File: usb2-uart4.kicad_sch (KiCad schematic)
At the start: 20 parts, among them U1 CH344Q, U13 TPNUP2202W1T2G, Y1 8MHz

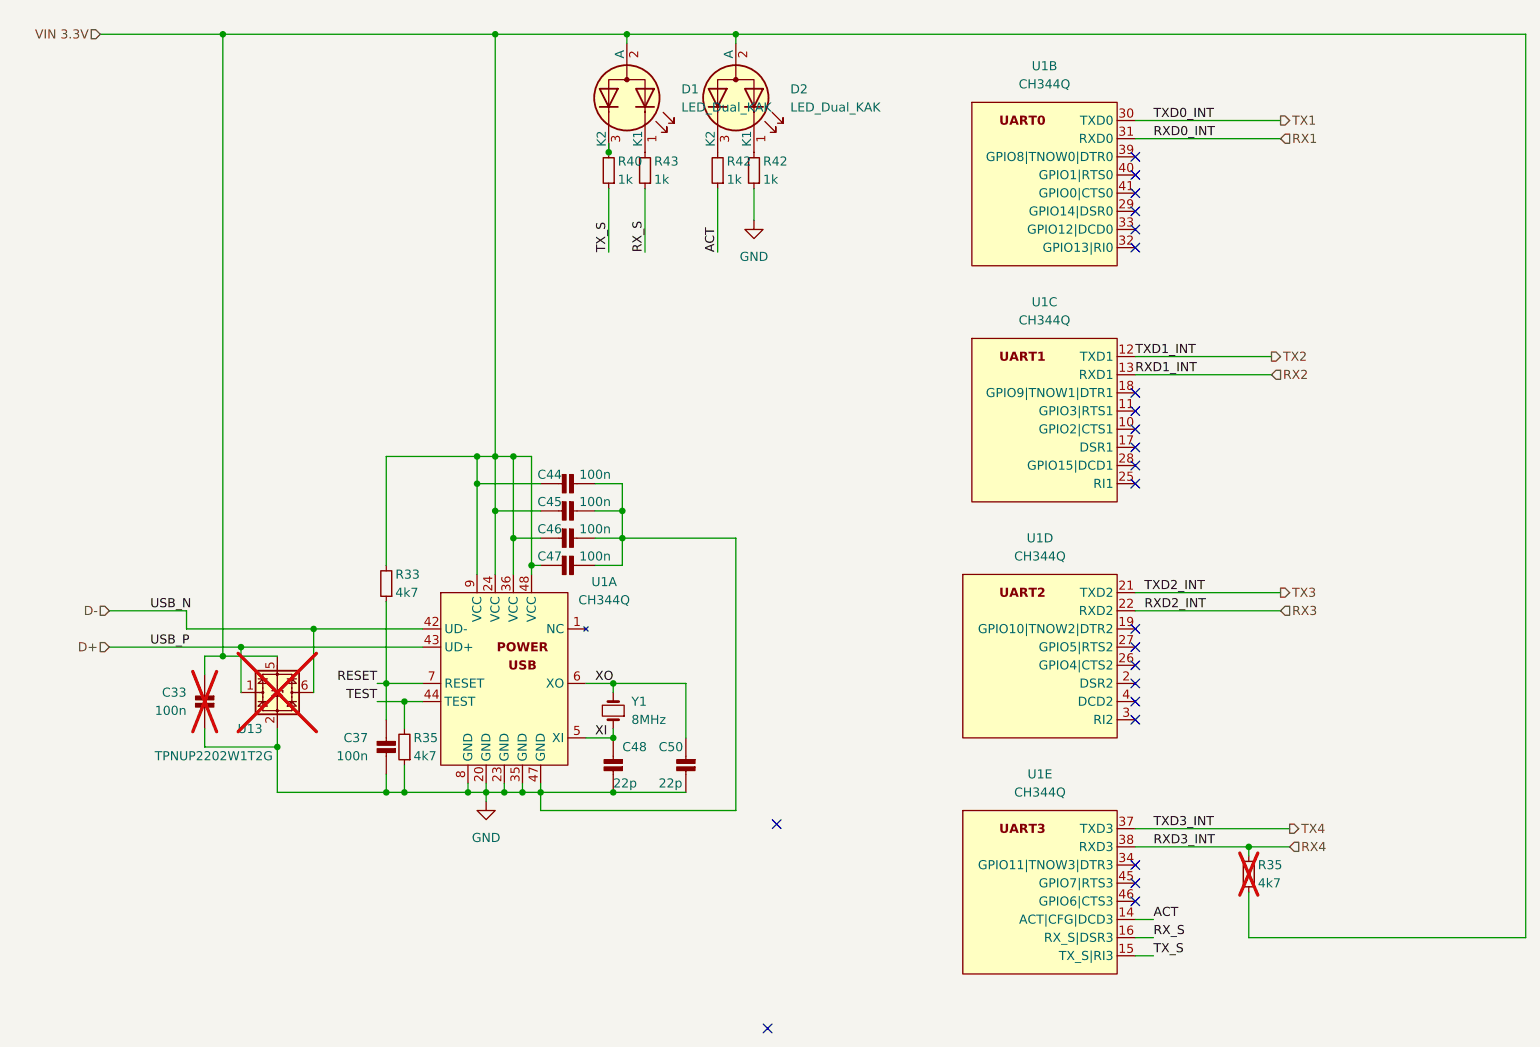
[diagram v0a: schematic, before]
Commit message: More feng shui
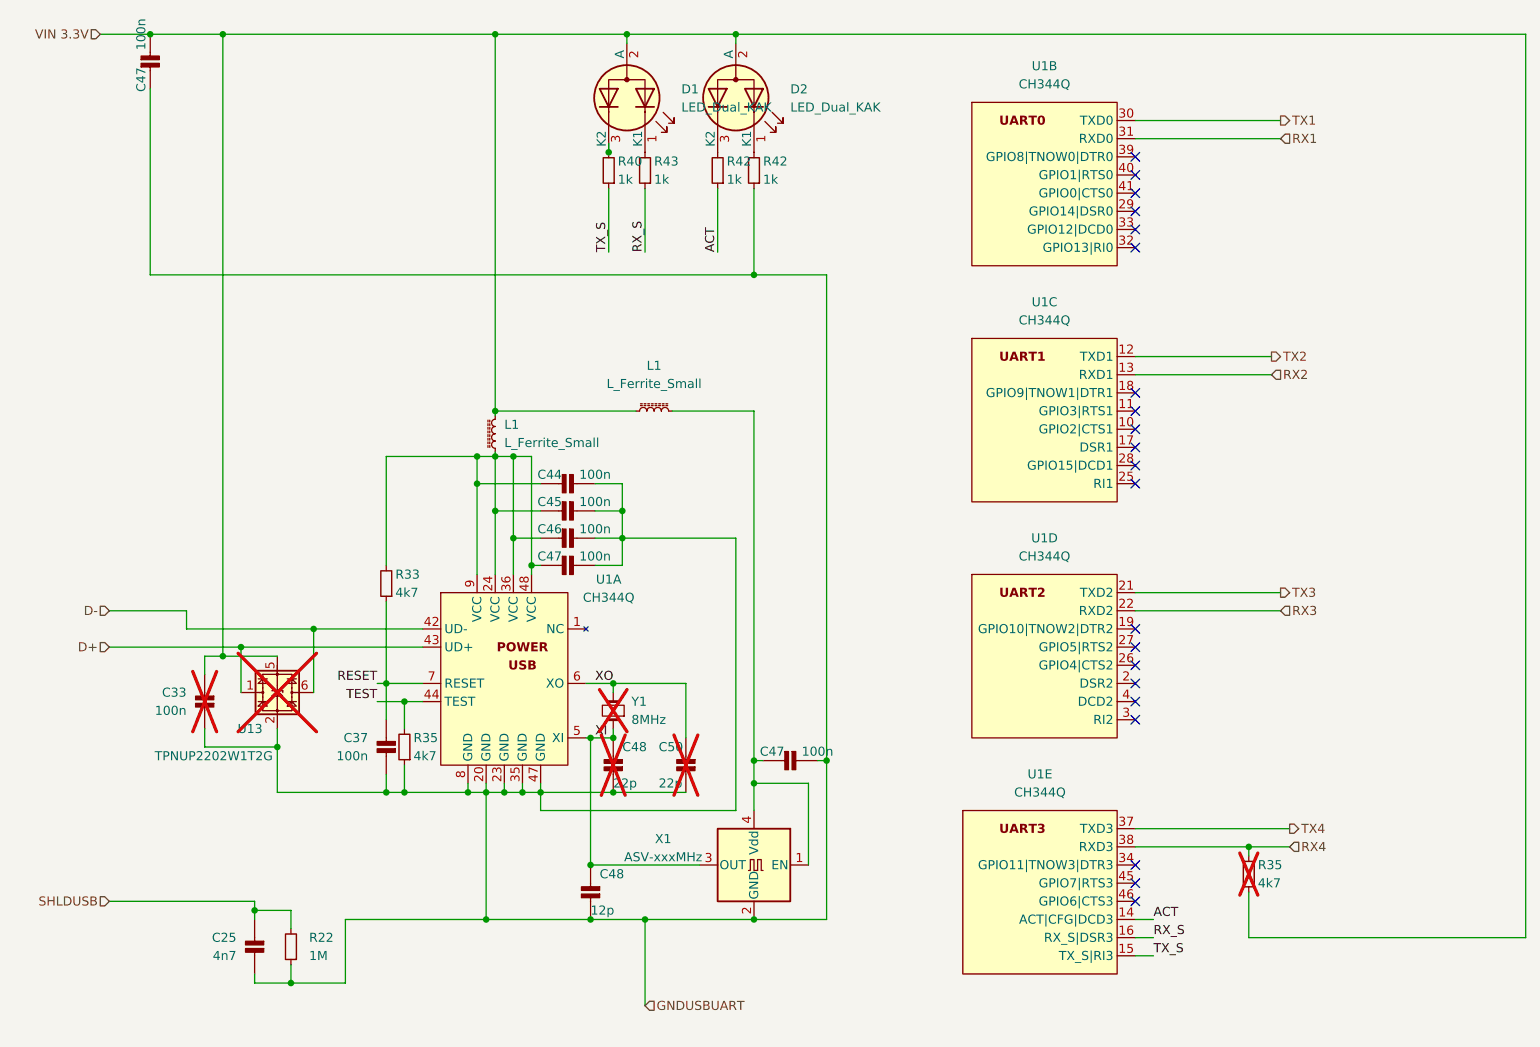
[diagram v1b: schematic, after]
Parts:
- added C25: 4n7, Capacitor_SMD:C_0805_2012Metric_Pad1.18x1.45mm_HandSolder, symbol H_passives:CAP_NP
- added C47 (x2): 100n, Capacitor_SMD:C_0805_2012Metric_Pad1.18x1.45mm_HandSolder, symbol H_passives:CAP_NP
- added C48: 12p, Capacitor_SMD:C_0805_2012Metric_Pad1.18x1.45mm_HandSolder, symbol H_passives:CAP_NP
- added L1 (x2): L_Ferrite_Small, Inductor_SMD:L_TDK_NLV25_2.5x2.0mm, symbol Device:L_Ferrite_Small
- added R22: 1M, Resistor_SMD:R_0805_2012Metric_Pad1.20x1.40mm_HandSolder, symbol Device:R_Small
- added X1: ASV-xxxMHz, Oscillator:Oscillator_SMD_Abracon_ASV-4Pin_7.0x5.1mm, symbol Oscillator:ASV-xxxMHz
- C37: footprint Capacitor_SMD:C_0603_1608Metric_Pad1.08x0.95mm_HandSolder -> Capacitor_SMD:C_0805_2012Metric_Pad1.18x1.45mm_HandSolder
- C48, C50: now not fitted; now left out of the parts list
- U1: symbol H_interface_esd:CH344Q -> isouart4:CH344Q
- Y1: footprint Crystal:Crystal_HC49-U_Vertical -> Crystal:Crystal_SMD_7050-4Pin_7.0x5.0mm; now not fitted; now left out of the parts list
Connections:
- net VIN 3.3V: now also C47.1, L1.1, L1.2; no longer C44.2, C45.2, C46.2, C47.2, R33.2, U1.24 (VCC), U1.36 (VCC), U1.48 (VCC), U1.9 (VCC)
- net XI: now also C48.2, X1.3 (OUT)
- net GND renamed GNDUSBUART
- net GNDUSBUART: now also C25.1, C47.1, C47.2, C48.1, R22.1, X1.2 (GND)
- new net: C44.2, C45.2, C46.2, C47.2, L1.1, R33.2, U1.24 (VCC), U1.36 (VCC), U1.48 (VCC), U1.9 (VCC)
- new net: C47.2, L1.2, X1.1 (EN), X1.4 (Vdd)
- new net SHLDUSB: C25.2, R22.2
- no-connect marks 23 -> 21
